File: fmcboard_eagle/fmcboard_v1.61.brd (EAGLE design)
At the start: 147 x 74 mm, 214 parts, among them IC1 OPA695IDR, IC10 LM358, IC11 7805TV, IC12 SN74AUC2G66DCTR, IC13 SN74AUC2G66DCTR, IC14 SN74AUC2G66DCTR, IC15 SN74AUC2G66DCTR, IC16 DAC7578SPWR, IC17 SN74AUC2G66DCTR, IC18 SN74AUC2G66DCTR, IC19 SN74AUC2G66DCTR, IC2 DAC7578SPWR, IC20 SN74AUC2G66DCTR, IC21 74AUP2GU04GW, IC22 74AUP2GU04GW, IC23 74AUP2GU04GW, IC24 74AUP2GU04GW, IC25 LM358, IC26 AMS1117-1.8, IC27 OPA699ID, IC3 LTC6229IMS8E#TRPBF, IC4 OPA695IDR, IC5 LTC6229IMS8E#TRPBF, IC6 OPA695IDR, IC7 OPA699ID, IC8 LM358, IC9 LM358, J1 8pin, J10 8pin, J11 8pin, J12 4p-2.54, J2 ASP-134604-01, J3 4p-2.54, J4 4p-2.54, J5 8pin, J6 4p-2.54, J7 4p-2.54, J8 4p-2.54, J9 8pin, U1 TXS0108EPWR, U2 STMICROELECTRONICS_L7905ACVST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

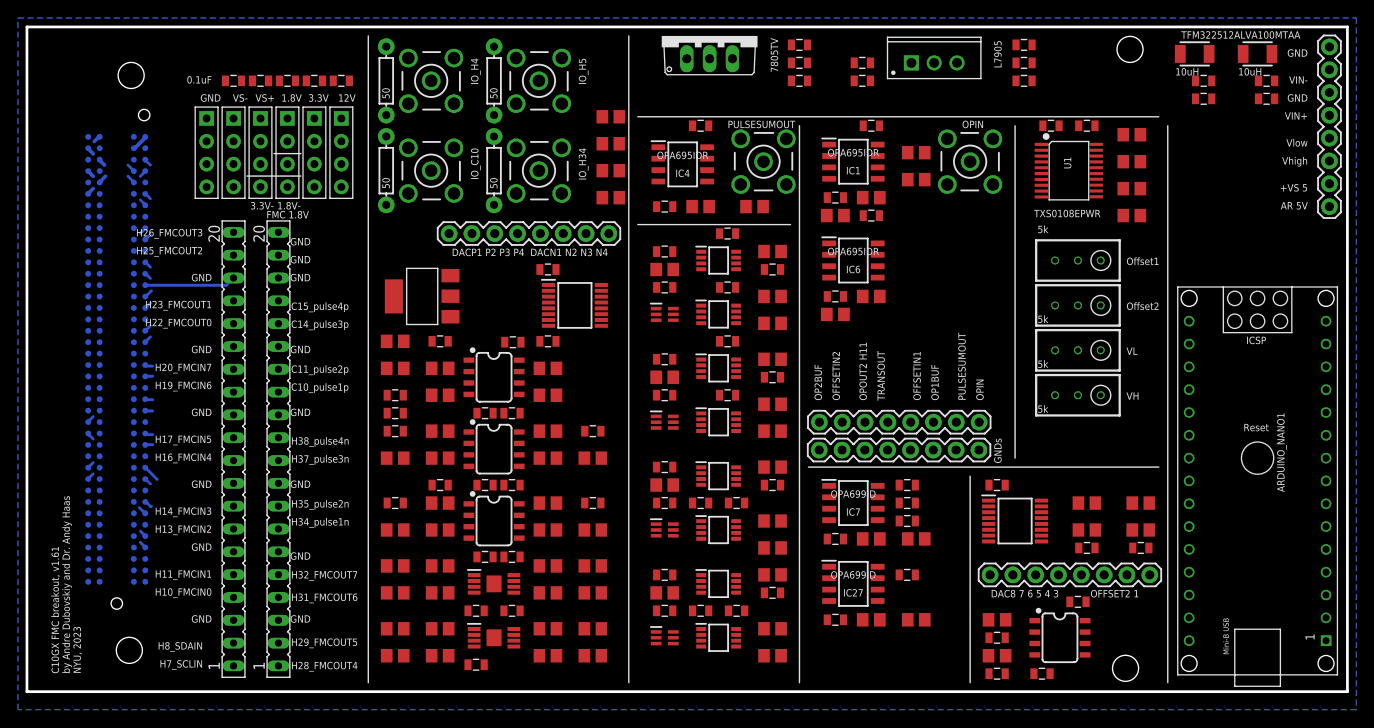
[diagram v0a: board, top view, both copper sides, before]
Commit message: routed
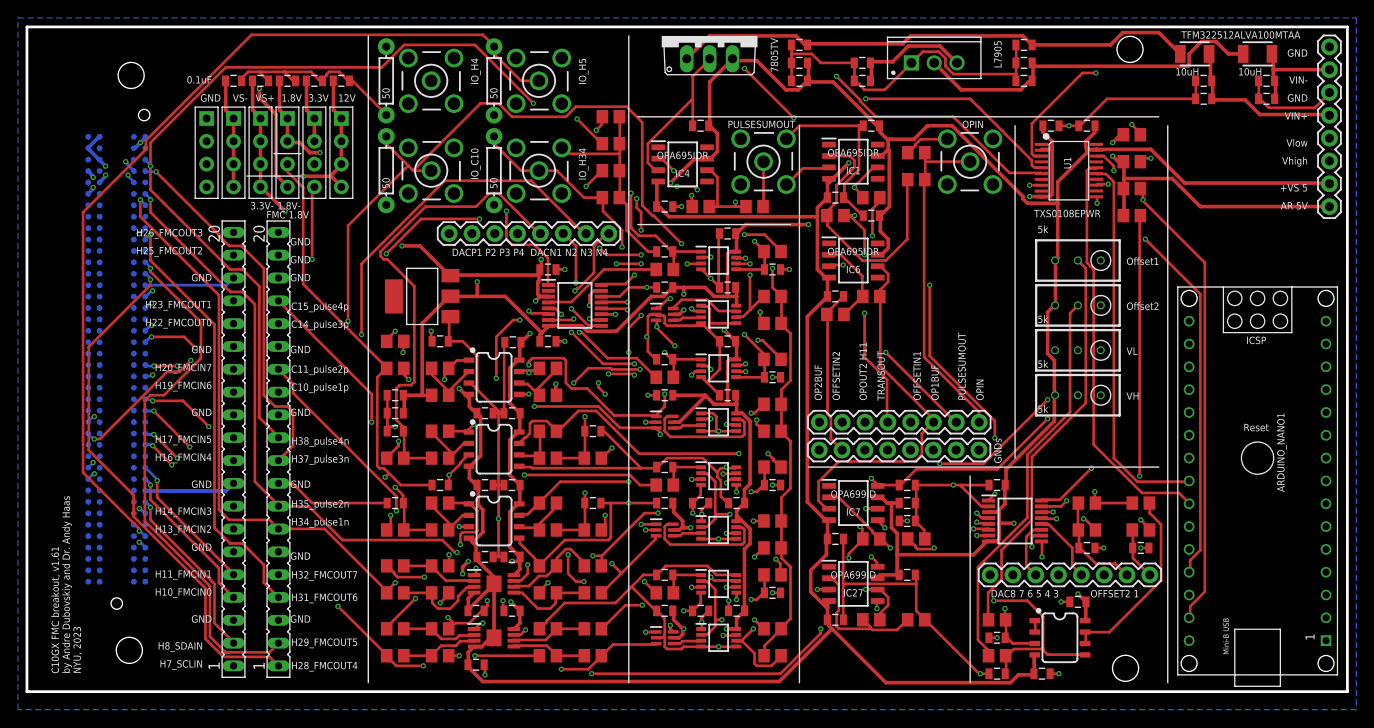
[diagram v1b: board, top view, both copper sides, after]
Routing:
- net GND: track 10.3 -> 520.5 mm, vias 0 -> 41
- net VS+: track 0.00 -> 330.6 mm, vias 0 -> 12
- net VS-: track 0.00 -> 319.3 mm, vias 0 -> 2
- net 1V8: track 0.00 -> 238.0 mm, vias 0 -> 10
- net SDAIN: track 0.91 -> 225.6 mm, vias 0 -> 2
- net SCLIN: track 0.94 -> 193.2 mm, vias 0 -> 4
- net AR_SCLIN2: track 0.00 -> 162.7 mm, vias 0 -> 5
- net H38: track 0.83 -> 157.3 mm, vias 0 -> 4
- net H37: track 0.80 -> 155.6 mm, vias 0 -> 5
- net H35: track 0.79 -> 149.4 mm, vias 0 -> 6
- net H34: track 0.82 -> 147.6 mm, vias 0 -> 4
- net 1V8-: track 0.00 -> 139.8 mm, vias 0 -> 7
- net AR_SDAIN2: track 0.00 -> 134.8 mm, vias 0 -> 5
- net OPOUT2_H11: track 1.86 -> 130.4 mm, vias 0 -> 4
- net C10: track 0.81 -> 128.3 mm, vias 0 -> 5
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
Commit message: routed
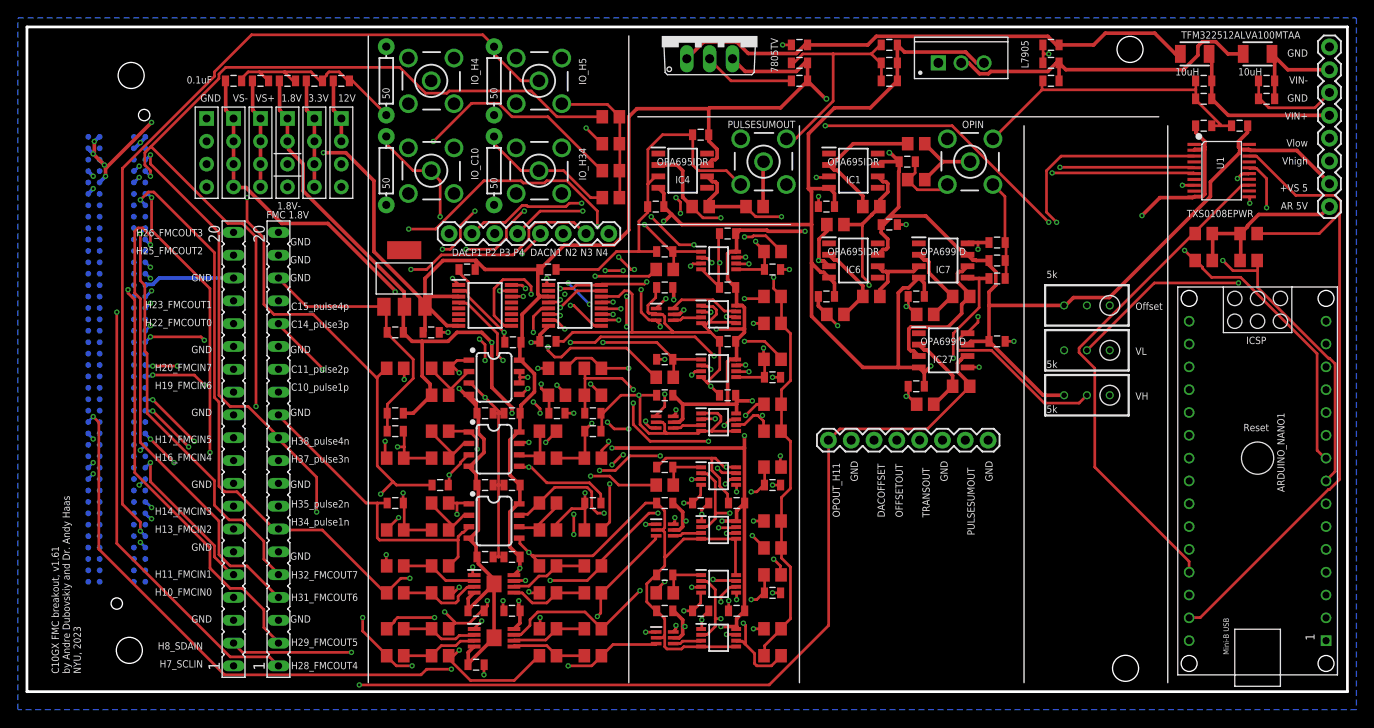
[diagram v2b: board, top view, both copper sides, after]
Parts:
- removed C11: 0.1uF, SparkFun-Passives:0805
- removed C32, C65: 1uF, SparkFun-Passives:0805
- removed IC25: LM358, SparkFun-IC-Amplifiers:SO08
- removed J10, J11: 8pin, SparkFun-Connectors:1X08
- removed R3: 100k, rcl:R0805
- removed R61, R79: 100, rcl:R0805
- removed R70, R73: 1k, rcl:R0805
- removed R_O1: 5k, resistor:RTRIM3296W
- moved C75 78.0 mm to (45.0, 40.0), turned to 0 degrees
- moved C25 72.0 mm to (96.0, 72.0), turned to 180 degrees
- moved R25 66.7 mm to (59.0, 36.0), turned to 180 degrees
- moved C9 63.7 mm to (49.0, 47.0)
- moved IC16 63.7 mm to (51.0, 43.0)
- moved C64 62.8 mm to (63.0, 31.0)
- moved R60 62.8 mm to (63.0, 33.0)
- moved R31 57.0 mm to (63.0, 36.0)
- moved C4 56.9 mm to (59.0, 31.0), turned to 0 degrees
- moved R17 56.9 mm to (59.0, 33.0), turned to 0 degrees
- moved C28 28.8 mm to (108.0, 48.0)
- moved C7 28.8 mm to (108.0, 50.0)
- moved C8 28.8 mm to (108.0, 46.0)
- moved IC7 28.8 mm to (102.0, 48.0)
- moved R6 28.8 mm to (104.0, 44.0), turned to 0 degrees
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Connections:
- net OPOUT1_H10 renamed H10
- removed net 3V3-: C32.2, J3.4, R79.1
- removed net DAC3: IC16.5, J10.3
- removed net DAC4: IC16.12, J10.4
- removed net DAC5: IC16.6, J10.5
- removed net DAC6: IC16.11, J10.6
- removed net DAC7: IC16.7, J10.7
- removed net DAC8: IC16.10, J10.8
- removed net DACOFFSET1: C64.2, J10.1, R60.2
- removed net DACOFFSET2: C65.1, J10.2, R31.2, R61.1
- removed net N$30: IC16.13, R61.2
- removed net N$36: IC10.7, R70.2, R79.2
- removed net N$37: IC10.6, R70.1, R73.1
- removed net N$8: R3.2, R_O1.2
- removed net OFFSETIN1: C11.1, IC25.3, J5.4, R3.1
- removed net OFFSETIN2: C4.1, IC25.5, J5.7, R17.1
- removed net OFFSETOUT1: IC25.1, IC25.2
- removed net OFFSETOUT2: IC25.6, IC25.7, R25.2
- removed net OPOUT2_H11: IC27.6, J2.H11, J5.6, R9.2, SV1.5
- new net DACOFFSET: C64.2, J5.6, R31.2, R60.2
- new net OFFSETIN: C4.1, IC10.5, R17.1
- new net OFFSETOUT: IC10.6, IC10.7, J5.5, R25.2
- new net OPOUT_H11: IC27.6, J2.H11, J5.8, R9.2, SV1.5
- net 3V3: now also J3.4; no longer R73.2
- net GND: now also J5.1, J5.3, J5.7; no longer C11.2, C32.1, C65.2, IC10.5, J11.1, J11.2, J11.3, J11.4, J11.5, J11.6, J11.7, J11.8
- net IO1: no longer J5.1
- net OP1BUF: no longer J5.3
- net OP2BUF: no longer J5.8
- net TRANSOUT: now also J5.4; no longer J5.5
- net VS+: no longer IC25.8, R_O1.3
- net VS-: no longer IC25.4, R_O1.1
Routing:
- net OPOUT_H11: track 0.00 -> 134.8 mm, vias 0 -> 2
- net OPOUT2_H11: track 130.4 -> 0.00 mm, vias 4 -> 0
- net DACLDAC: track 98.3 -> 12.6 mm, vias 4 -> 2
- net DACCLR: track 102.6 -> 20.8 mm, vias 6 -> 3
- net C15: track 90.5 -> 166.2 mm, vias 5 -> 4
- net N$2: track 44.1 -> 115.4 mm, vias 0 -> 7
- net VS-: track 319.3 -> 259.7 mm, vias 2 -> 4
- net OFFSETIN2: track 53.4 -> 0.00 mm, vias 1 -> 0
- net OFFSETOUT: track 0.00 -> 51.4 mm, vias 0 -> 4
- net SDAIN: track 225.6 -> 174.6 mm, vias 2 -> 3
- net AR_SCLIN2: track 162.7 -> 117.4 mm, vias 5 -> 6
- net N$8: track 44.9 -> 0.00 mm
- net DACOFFSET: track 0.00 -> 43.4 mm, vias 0 -> 3
- net OFFSETIN1: track 34.1 -> 0.00 mm, vias 1 -> 0
- net 3V3: track 80.1 -> 46.5 mm, vias 3 -> 5
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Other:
- board text added: "DACOFFSET"
- board text added: "OFFSETOUT"
- board text added: "OPOUT_H11"
- board text added: "Offset"
- board text removed: "3.3V-"
- board text removed: "DAC8 7 6 5 4 3 OFFSET2 1"
- board text removed: "GNDs"
- board text removed: "OFFSETIN1"
- board text removed: "OFFSETIN2"
- board text removed: "OP1BUF"
- board text removed: "OP2BUF"
- board text removed: "OPIN"
- board text removed: "OPOUT2 H11"
- board text removed: "Offset1"
- board text removed: "Offset2"
